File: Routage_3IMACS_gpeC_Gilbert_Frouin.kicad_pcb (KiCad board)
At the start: 2 copper layers, 52 parts, among them J2 Conn_01x02, J3 Conn_01x03, Q1 2N2907, Q10 TIP31, Q11 BD138, Q12 TIP31, Q13 2N2222, Q2 2N2907, Q3 2N2907, Q4 2N2222, Q5 2N2222, Q6 2N2907, Q7 2N2907, Q8 BD139, Q9 BD139, U1 Relay_1CT, U2 Jack_Mono

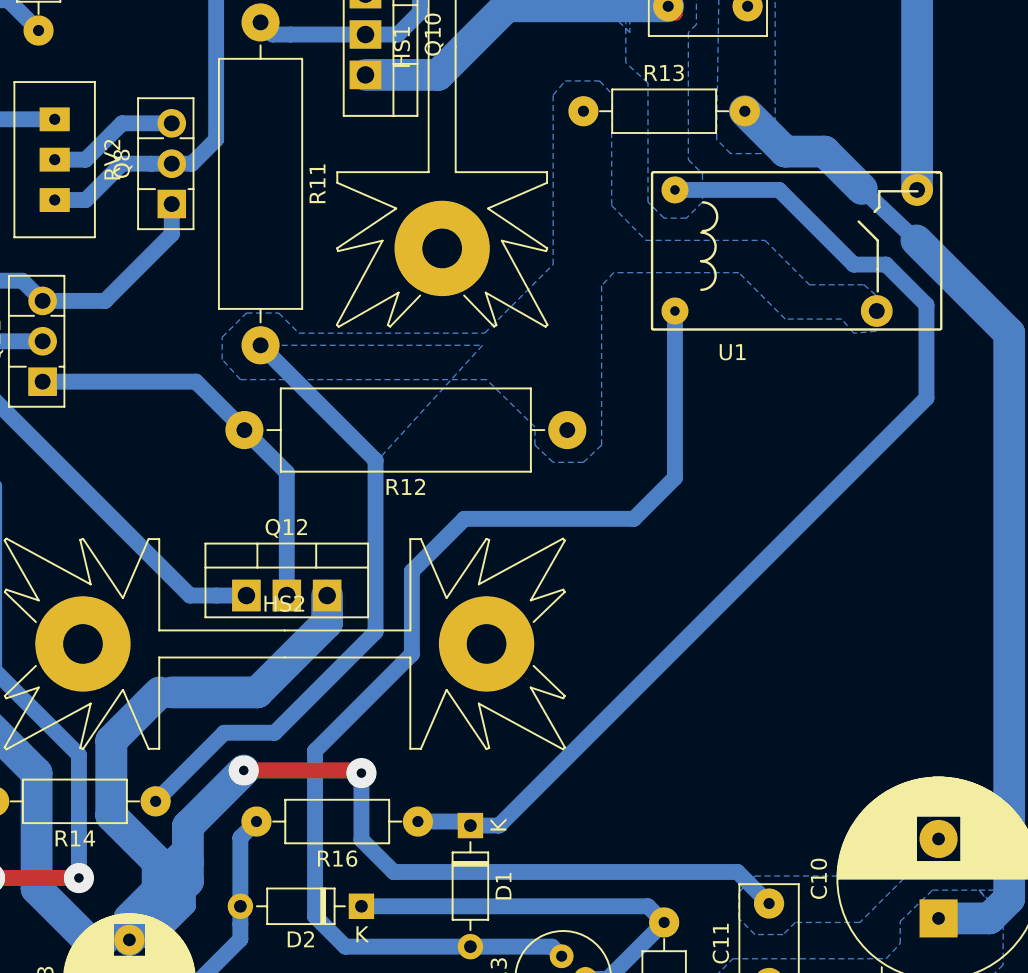
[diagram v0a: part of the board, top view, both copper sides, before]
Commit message: etape2
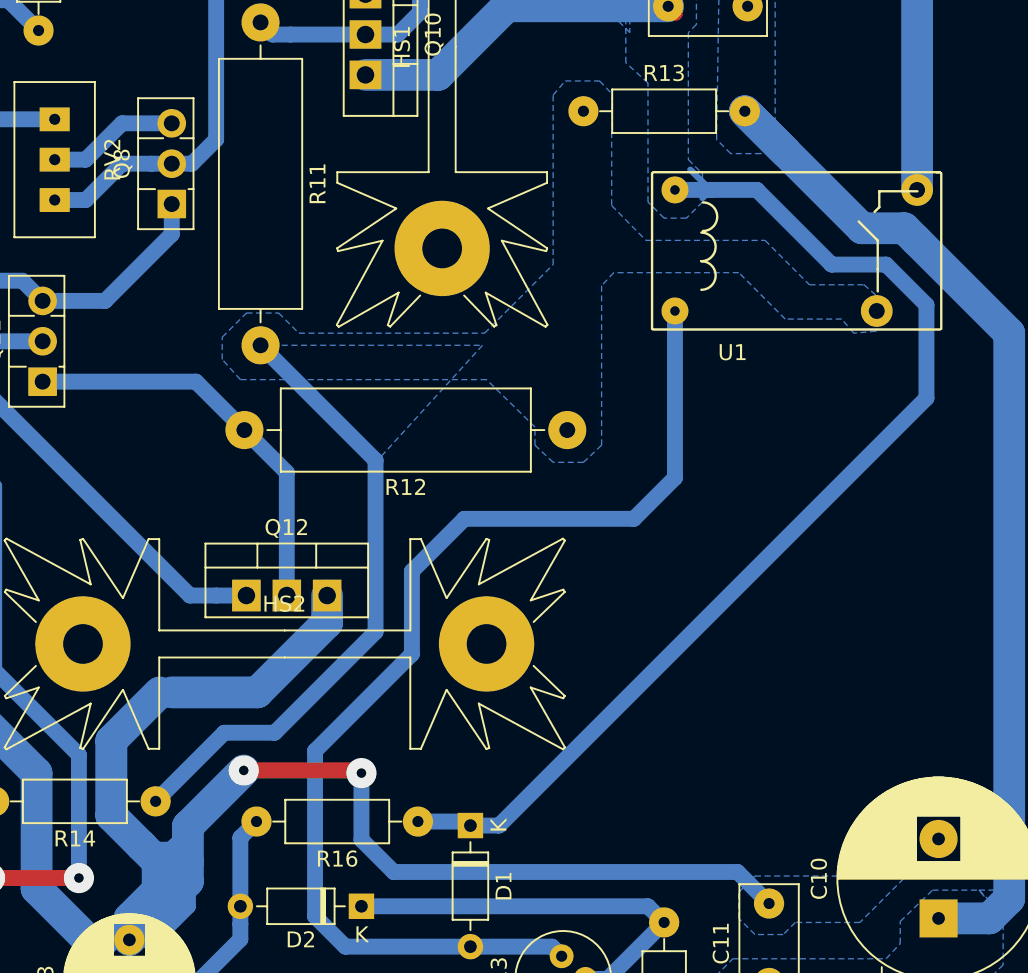
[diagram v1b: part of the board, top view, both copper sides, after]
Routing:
- net -12V: track 212.8 -> 218.3 mm
- net GND: track 136.7 -> 140.3 mm
- net +12V: track 90.6 -> 93.2 mm
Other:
- board text added: "Valentin Gilbert - Mathis Frouin Routage amplificateur audio 3IMACS 2020"
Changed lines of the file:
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@@
   (general
     (thickness 1.6)
-    (drawings 4)
-    (tracks 262)
+    (drawings 5)
+    (tracks 272)
     (zones 0)
     (modules 52)
@@
   )
   (setup
-    (last_trace_width 2)
+    (last_trace_width 0.4)
     (user_trace_width 0.4)
     (user_trace_width 0.5)
@@
       (net 2 /JC1))
   )
+  (gr_text "Valentin Gilbert - Mathis Frouin\nRoutage amplificateur audio\n3IMACS 2020" (at 144.653 101.473 90) (layer Margin)
+    (effects (font (size 1.5 1.5) (thickness 0.3)))
+  )
   (gr_line (start 151.148 77.724) (end 151.148 177.724) (layer F.SilkS) (width 0.12))
   (gr_line (start 41.148 177.724) (end 41.148 77.724) (layer F.SilkS) (width 0.12))
@@
   (segment (start 94.701179 154.772179) (end 101.940179 154.772179) (width 1) (layer F.Cu) (net 5))
   (segment (start 89.027 160.274) (end 90.043 160.274) (width 1) (layer B.Cu) (net 5))
-  (segment (start 86.868 158.115) (end 89.027 160.274) (width 1) (layer B.Cu) (net 5))
   (segment (start 91.186 159.131) (end 91.186 158.287358) (width 1) (layer B.Cu) (net 5))
   (segment (start 90.043 160.274) (end 91.186 159.131) (width 1) (layer B.Cu) (net 5))
@@
   (segment (start 87.503 164.090498) (end 89.281 162.312498) (width 2) (layer B.Cu) (net 5))
   (segment (start 87.503 165.434) (end 87.503 164.090498) (width 2) (layer B.Cu) (net 5))
-  (segment (start 89.281 160.528) (end 86.36 157.607) (width 2) (layer B.Cu) (net 5))
   (segment (start 86.36 152.908) (end 89.408 149.86) (width 2) (layer B.Cu) (net 5))
   (segment (start 86.36 157.607) (end 86.36 152.908) (width 2) (layer B.Cu) (net 5))
@@
   (segment (start 95.553002 149.86) (end 99.949 145.464002) (width 2) (layer B.Cu) (net 5))
   (segment (start 90.17 149.86) (end 89.408 149.86) (width 1) (layer B.Cu) (net 5))
+  (segment (start 88.646 159.893) (end 89.580358 159.893) (width 0.5) (layer B.Cu) (net 5))
+  (segment (start 88.646 159.893) (end 89.027 160.274) (width 1) (layer B.Cu) (net 5))
+  (segment (start 86.868 158.115) (end 88.646 159.893) (width 1) (layer B.Cu) (net 5))
+  (segment (start 90.043 159.512) (end 90.424 159.131) (width 0.5) (layer B.Cu) (net 5))
+  (segment (start 88.265 159.512) (end 90.043 159.512) (width 0.5) (layer B.Cu) (net 5))
+  (segment (start 89.281 160.528) (end 88.265 159.512) (width 2) (layer B.Cu) (net 5))
+  (segment (start 88.265 159.512) (end 86.36 157.607) (width 2) (layer B.Cu) (net 5))
+  (segment (start 89.580358 159.893) (end 90.424 159.131) (width 0.5) (layer B.Cu) (net 5))
+  (segment (start 90.424 159.131) (end 91.186 158.287358) (width 0.5) (layer B.Cu) (net 5))
   (segment (start 94.488 164.45337) (end 94.488 163.322) (width 1) (layer B.Cu) (net 6))
   (segment (start 94.488 165.399) (end 94.488 164.45337) (width 1) (layer B.Cu) (net 6))
@@
   (segment (start 114.708 170.842) (end 110.998 174.552) (width 1) (layer B.Cu) (net 7))
   (segment (start 126.238 113.284) (end 128.778 115.824) (width 2) (layer B.Cu) (net 7))
-  (segment (start 131.25149 115.824) (end 133.604 118.17651) (width 2) (layer B.Cu) (net 7))
-  (segment (start 128.778 115.824) (end 131.25149 115.824) (width 2) (layer B.Cu) (net 7))
   (segment (start 142.875 127.254) (end 137.033 121.412) (width 2) (layer B.Cu) (net 7))
   (segment (start 141.63 164.084) (end 142.875 162.839) (width 2) (layer B.Cu) (net 7))
   (segment (start 138.43 164.084) (end 141.63 164.084) (width 2) (layer B.Cu) (net 7))
   (segment (start 142.875 162.839) (end 142.875 127.254) (width 2) (layer B.Cu) (net 7))
-  (segment (start 133.604 118.17651) (end 137.033 121.412) (width 1) (layer B.Cu) (net 7))
+  (segment (start 133.604 120.65) (end 126.238 113.284) (width 2) (layer B.Cu) (net 7))
+  (segment (start 137.033 121.412) (end 136.271 120.65) (width 2) (layer B.Cu) (net 7))
+  (segment (start 136.271 120.65) (end 133.604 120.65) (width 2) (layer B.Cu) (net 7))
   (segment (start 44.323 136.144) (end 43.688 135.509) (width 1) (layer F.Cu) (net 8))
   (segment (start 121.839 107.107) (end 121.412 106.68) (width 1) (layer F.Cu) (net 8))
@@
   (segment (start 108.712 157.988) (end 108.966 158.242) (width 1) (layer B.Cu) (net 8))
   (segment (start 105.664 157.988) (end 108.712 157.988) (width 1) (layer B.Cu) (net 8))
-  (segment (start 110.766 158.242) (end 108.966 158.242) (width 1) (layer B.Cu) (net 8))
-  (segment (start 137.668 131.34) (end 110.766 158.242) (width 1) (layer B.Cu) (net 8))
-  (segment (start 121.839 118.237) (end 128.397 118.237) (width 1) (layer B.Cu) (net 8))
-  (segment (start 128.397 118.237) (end 133.096 122.936) (width 1) (layer B.Cu) (net 8))
-  (segment (start 133.096 122.936) (end 135.128 122.936) (width 1) (layer B.Cu) (net 8))
-  (segment (start 137.668 125.476) (end 137.668 131.34) (width 1) (layer B.Cu) (net 8))
-  (segment (start 135.128 122.936) (end 137.668 125.476) (width 1) (layer B.Cu) (net 8))
   (segment (start 106.934 110.998) (end 111.252 106.68) (width 2) (layer B.Cu) (net 8))
   (segment (start 102.362 110.998) (end 106.934 110.998) (width 2) (layer B.Cu) (net 8))
   (segment (start 111.252 106.68) (end 121.412 106.68) (width 2) (layer B.Cu) (net 8))
+  (segment (start 121.839 118.237) (end 124.079 118.237) (width 1) (layer B.Cu) (net 8))
+  (segment (start 123.571 118.745) (end 124.079 118.237) (width 0.4) (layer B.Cu) (net 8))
+  (segment (start 124.079 118.237) (end 122.809 116.967) (width 0.4) (layer B.Cu) (net 8))
+  (segment (start 110.766 158.242) (end 108.966 158.242) (width 1) (layer B.Cu) (net 8))
+  (segment (start 137.668 131.34) (end 110.766 158.242) (width 1) (layer B.Cu) (net 8))
+  (segment (start 127 118.237) (end 131.699 122.936) (width 1) (layer B.Cu) (net 8))
+  (segment (start 124.079 118.237) (end 127 118.237) (width 1) (layer B.Cu) (net 8))
+  (segment (start 135.128 122.936) (end 137.668 125.476) (width 1) (layer B.Cu) (net 8))
+  (segment (start 131.699 122.936) (end 135.128 122.936) (width 1) (layer B.Cu) (net 8))
+  (segment (start 137.668 125.476) (end 137.668 131.34) (width 1) (layer B.Cu) (net 8))
   (segment (start 114.106 165.862) (end 114.708 166.464) (width 1) (layer B.Cu) (net 9))
   (segment (start 108.966 165.862) (end 114.106 165.862) (width 1) (layer B.Cu) (net 9))
